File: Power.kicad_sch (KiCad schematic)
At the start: 25 parts, among them J1 Power Input, U506 74LS03, U507 74LS32, U508 74LS04, U602 74LS04, U603 74LS00, U604 74LS04, U605 74LS32, U606 74LS00, U607 74LS74, U612 74LS00

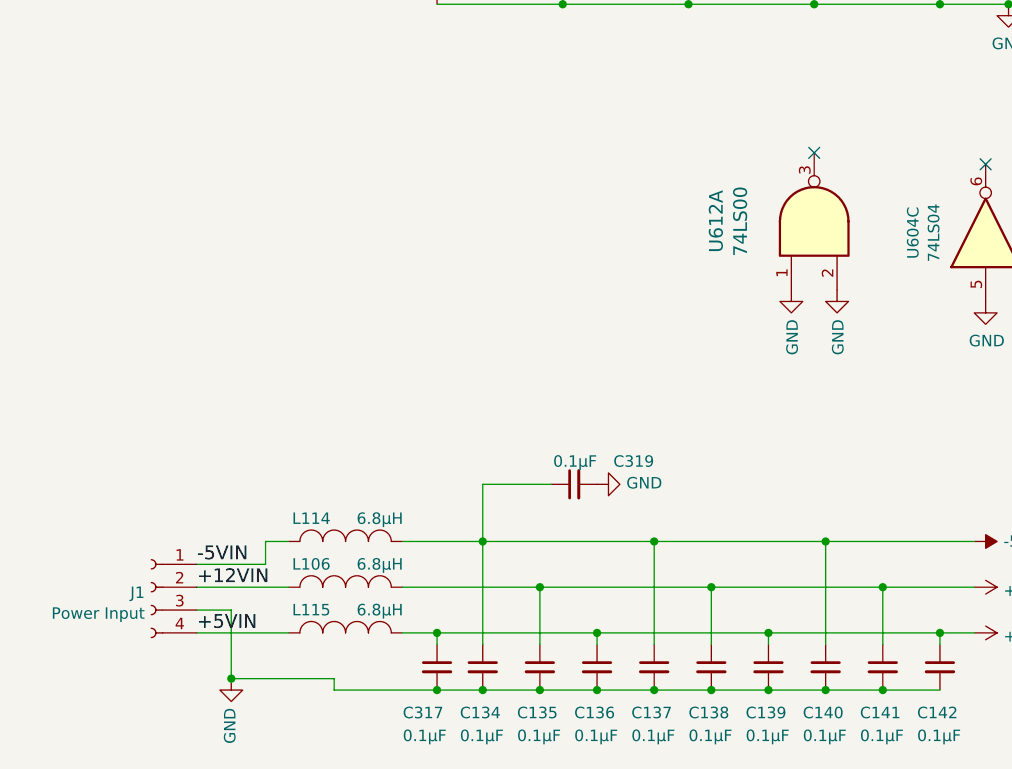
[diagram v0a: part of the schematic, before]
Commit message: Update to KiCAD 9
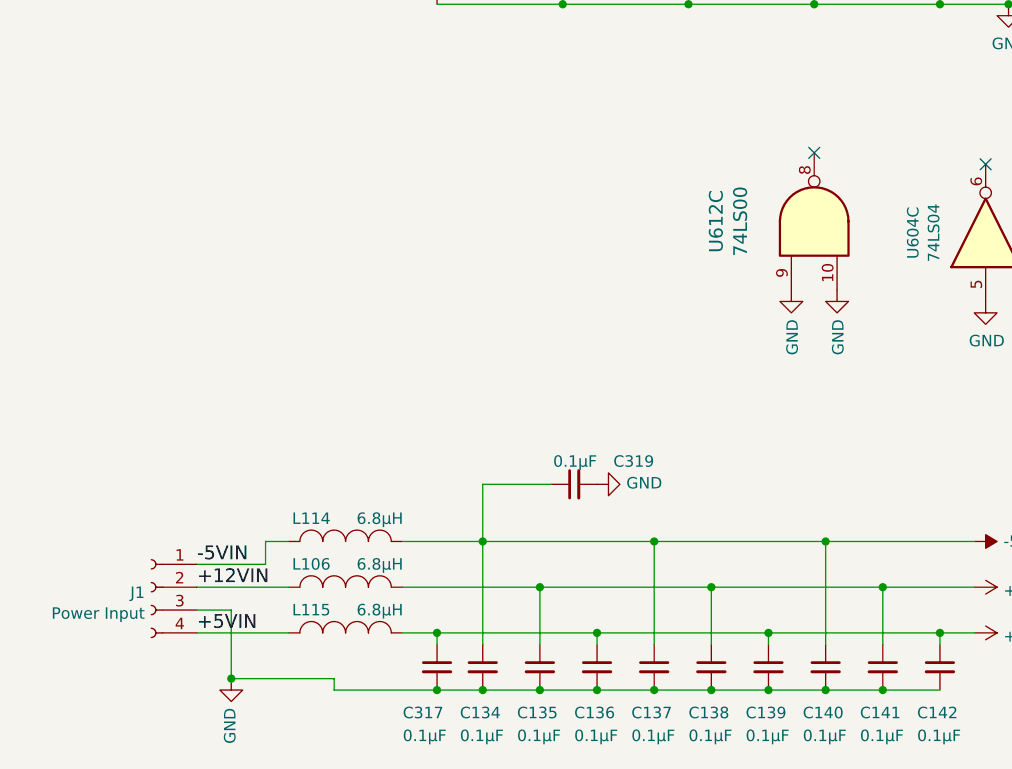
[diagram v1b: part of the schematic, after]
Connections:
- net GND: now also U612.10, U612.9; no longer U612.1, U612.2
